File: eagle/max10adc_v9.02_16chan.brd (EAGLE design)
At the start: 157 x 79 mm, 425 parts, among them IC1 MAX11105AUT+T, IC10 MAX11105AUT+T, IC11 MAX11105AUT+T, IC12 MAX11105AUT+T, IC13 MAX11105AUT+T, IC14 MAX11105AUT+T, IC15 MAX11105AUT+T, IC16 MAX11105AUT+T, IC2 MAX11105AUT+T, IC21 MAX11105AUT+T, IC22 MAX11105AUT+T, IC23 MAX11105AUT+T, IC24 MAX11105AUT+T, IC3 MAX11105AUT+T, IC4 MAX11105AUT+T, IC9 MAX11105AUT+T, K1 AQY21SOP, K10 AQY21SOP, K11 AQY21SOP, K12 AQY21SOP, K13 AQY21SOP, K14 AQY21SOP, K15 AQY21SOP, K16 AQY21SOP, K21 AQY21SOP, K22 AQY21SOP, K23 AQY21SOP, K24 AQY21SOP, K3 AQY21SOP, K5 AQY21SOP, K6 AQY21SOP, K9 AQY21SOP, U340G CH340G, Y1 ABL-12.000MHZ-B2

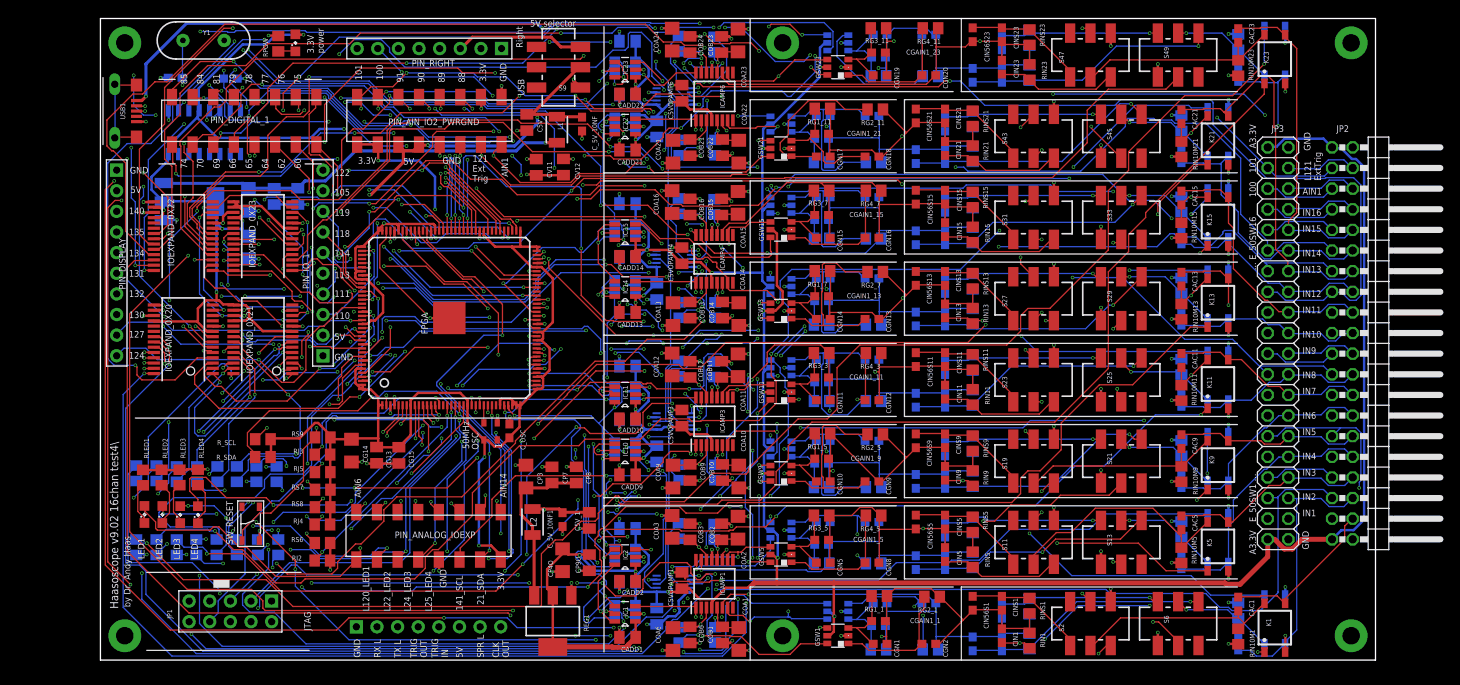
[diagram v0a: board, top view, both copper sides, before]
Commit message: back connectors
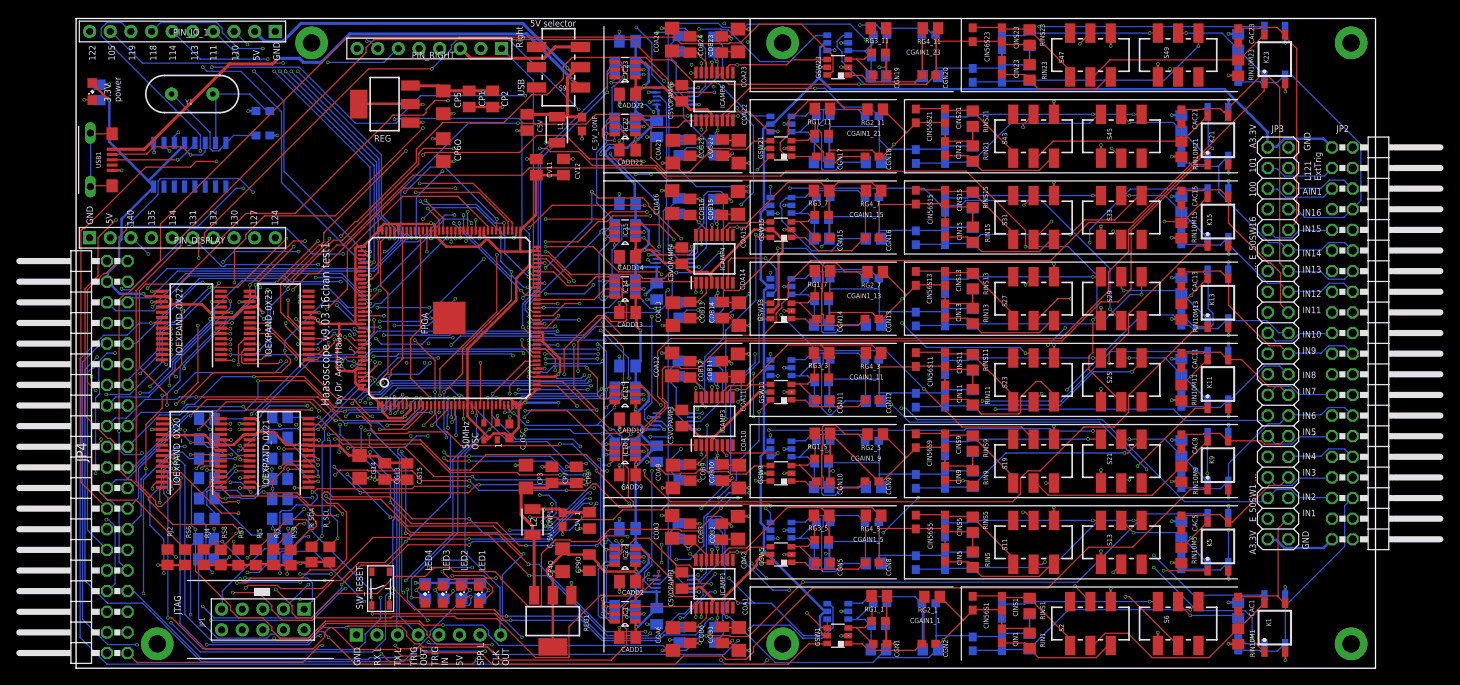
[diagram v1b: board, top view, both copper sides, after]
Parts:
- removed PIN_AIN_IO2_PWRGND, PIN_ANALOG_IOEXP, PIN_DIGITAL_1: 15-91-2160, pinhead+:2X08_SMT
- added JP4: (no value), pinhead:2X20/90
- moved RLED1 43.8 mm to (34.8, -3.47), flipped to the bottom
- moved LED1 42.3 mm to (34.6, -3.93), turned to 270 degrees
- moved RLED2 39.5 mm to (32.5, -3.48), flipped to the bottom
- moved LED2 38.1 mm to (32.4, -3.92), turned to 270 degrees
- moved RLED3 35.4 mm to (30.3, -3.49), flipped to the bottom
- moved LED3 33.8 mm to (30.2, -3.91), turned to 270 degrees
- moved PIN_IO_1 33.3 mm to (-1.90, 65.4), turned to 270 degrees
- moved RLED4 31.3 mm to (28.0, -3.50), flipped to the bottom
- moved LED4 29.7 mm to (28.0, -3.90), turned to 270 degrees
- moved CP1 26.8 mm to (33.4, 57.1), flipped to the top
- moved CP5 26.8 mm to (30.2, 56.7), flipped to the top
- moved CP6O 26.8 mm to (30.2, 50.8), flipped to the top
- moved REG 26.8 mm to (23.0, 56.5), flipped to the top
- moved CP2 26.8 mm to (36.3, 57.1), flipped to the top
- moved LEDPOW 25.7 mm to (-13.0, 58.0)
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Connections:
- net +3V3: now also JP4.38; no longer PIN_AIN_IO2_PWRGND.14, PIN_AIN_IO2_PWRGND.16, PIN_AIN_IO2_PWRGND.3, PIN_ANALOG_IOEXP.15
- net +5V: no longer PIN_AIN_IO2_PWRGND.10, PIN_AIN_IO2_PWRGND.12
- net A10: now also JP4.23; no longer PIN_ANALOG_IOEXP.8
- net A11: now also JP4.18; no longer PIN_ANALOG_IOEXP.10
- net A12: now also JP4.20; no longer PIN_ANALOG_IOEXP.12
- net A13: now also JP4.22; no longer PIN_ANALOG_IOEXP.14
- net A14: now also JP4.24; no longer PIN_ANALOG_IOEXP.16
- net A6: now also JP4.17; no longer PIN_ANALOG_IOEXP.2
- net A7: now also JP4.19; no longer PIN_ANALOG_IOEXP.4
- net A8: now also JP4.21; no longer PIN_ANALOG_IOEXP.6
- net AIN1: now also JP4.39; no longer PIN_AIN_IO2_PWRGND.2
- net D0C: now also JP4.1; no longer PIN_DIGITAL_1.1
- net D0D: now also JP4.2; no longer PIN_DIGITAL_1.2
- net D1C: now also JP4.3; no longer PIN_DIGITAL_1.3
- net D1D: now also JP4.4; no longer PIN_DIGITAL_1.4
- net D2C: now also JP4.5; no longer PIN_DIGITAL_1.5
- net D2D: now also JP4.6; no longer PIN_DIGITAL_1.6
- net D3C: now also JP4.7; no longer PIN_DIGITAL_1.7
- net D3D: now also JP4.8; no longer PIN_DIGITAL_1.8
- net D4C: now also JP4.9; no longer PIN_DIGITAL_1.9
- net D4D: now also JP4.10; no longer PIN_DIGITAL_1.10
- net D5C: now also JP4.11; no longer PIN_DIGITAL_1.11
- net D5D: now also JP4.12; no longer PIN_DIGITAL_1.12
- net D6C: now also JP4.13; no longer PIN_DIGITAL_1.13
- net D6D: now also JP4.14; no longer PIN_DIGITAL_1.14
- net D7C: now also JP4.15; no longer PIN_DIGITAL_1.15
- net D7D: now also JP4.16; no longer PIN_DIGITAL_1.16
- net GND: now also JP4.40; no longer PIN_AIN_IO2_PWRGND.1, PIN_AIN_IO2_PWRGND.6, PIN_AIN_IO2_PWRGND.8, PIN_ANALOG_IOEXP.9
- net IO_100: now also JP4.33; no longer PIN_AIN_IO2_PWRGND.13
- net IO_101: now also JP4.35; no longer PIN_AIN_IO2_PWRGND.15
- net IO_CLK_88: now also JP4.25; no longer PIN_AIN_IO2_PWRGND.5
- net IO_CLK_89: now also JP4.27; no longer PIN_AIN_IO2_PWRGND.7
- net IO_CLK_90: now also JP4.29; no longer PIN_AIN_IO2_PWRGND.9
- net IO_CLK_91: now also JP4.31; no longer PIN_AIN_IO2_PWRGND.11
- net L120_LED1: now also JP4.36; no longer PIN_ANALOG_IOEXP.1
- net L121: now also JP4.37; no longer PIN_AIN_IO2_PWRGND.4
- net L141_SCL: now also JP4.28; no longer PIN_ANALOG_IOEXP.11
- net L21_SDA: now also JP4.26; no longer PIN_ANALOG_IOEXP.13
- net L22_LED2: now also JP4.34; no longer PIN_ANALOG_IOEXP.3
- net L24_LED3: now also JP4.32; no longer PIN_ANALOG_IOEXP.5
- net L25_LED4: now also JP4.30; no longer PIN_ANALOG_IOEXP.7
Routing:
- net E_50SW5: track 251.9 -> 158.2 mm, vias 2 -> 9
- net D4C: track 53.1 -> 131.8 mm, vias 4 -> 3
- net E_50SW7: track 225.7 -> 152.4 mm, vias 8 -> 3
- net E_50SW2: track 229.3 -> 157.8 mm, vias 7 -> 4
- net E_50SW4: track 236.4 -> 165.6 mm, vias 4 -> 3
- net L24_LED3: track 55.9 -> 126.3 mm, vias 6 -> 3
- net E_50SW3: track 227.4 -> 157.2 mm, vias 7 -> 5
- net E_50SW11: track 205.5 -> 143.0 mm, vias 6 -> 3
- net D3D: track 42.5 -> 105.0 mm, vias 4 -> 6
- net E_50SW14: track 206.4 -> 145.7 mm, vias 6 -> 3
- net L22_LED2: track 54.7 -> 114.1 mm, vias 5 -> 3
- net E_50SW12: track 203.0 -> 144.7 mm, vias 4 -> 3
- net +3V3: track 379.2 -> 321.0 mm
- net D7D: track 39.6 -> 96.3 mm
- net D3C: track 59.3 -> 115.7 mm, vias 3 -> 4
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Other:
- board size 157 x 79 mm -> 160 x 80 mm
- board text added: "Haasoscope v9.03 16chan test1"
- board text removed: "121 Ext Trig"
- board text removed: "141_SCL"
- board text removed: "21_SDA"
- board text removed: "22pF"
- board text removed: "3.3V"
- board text removed: "60"
- board text removed: "62"
- board text removed: "64"
- board text removed: "65"
- board text removed: "66"
- board text removed: "69"
- board text removed: "70"
- board text removed: "74"
- board text removed: "75"
- board text removed: "76"
- board text removed: "77"
- board text removed: "78"
- board text removed: "79"
- board text removed: "81"
- board text removed: "84"
- board text removed: "85"
- board text removed: "88"
- board text removed: "89"
- board text removed: "90"
- board text removed: "91"
- board text removed: "AIN14"
- board text removed: "AIN6"
- board text removed: "Haasoscope v9.02 16chan test4\"
- board text removed: "L120_LED1"
- board text removed: "L22_LED2"
- board text removed: "L24_LED3"
- board text removed: "L25_LED4"
